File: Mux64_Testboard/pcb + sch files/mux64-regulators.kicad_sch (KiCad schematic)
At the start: 25 parts, among them J10 Conn_01x24, J7 Conn_01x24, J8 Conn_01x24, J9 Conn_01x24, U1 LD1117AS12TR, U2 MAX6070

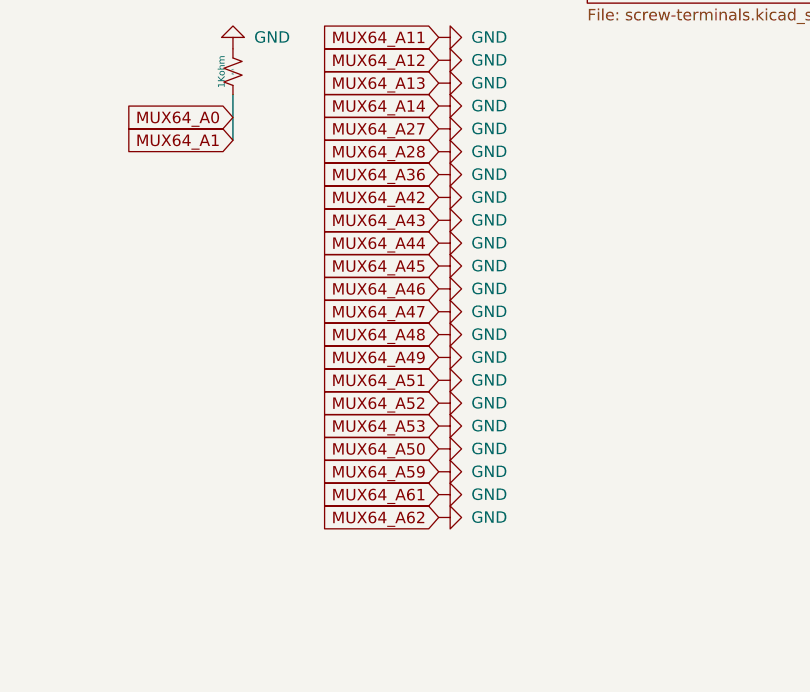
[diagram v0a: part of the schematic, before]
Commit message: Completed v2
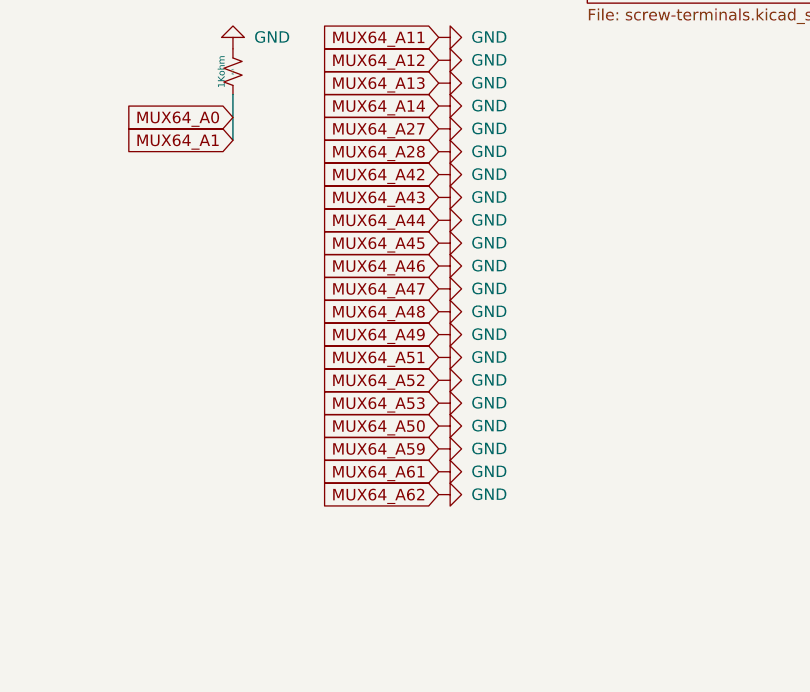
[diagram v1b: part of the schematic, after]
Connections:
- net GND: no longer J9.3 (Pin_3)
- new net MUX64_A36: J9.3 (Pin_3)
